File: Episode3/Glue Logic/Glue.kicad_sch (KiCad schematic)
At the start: 17 parts, among them U10 ATF750C, U11 ATF22V10, U7 ATF22V10C, U8 ATF22V10, U9 ATF750C, X1 16MHz

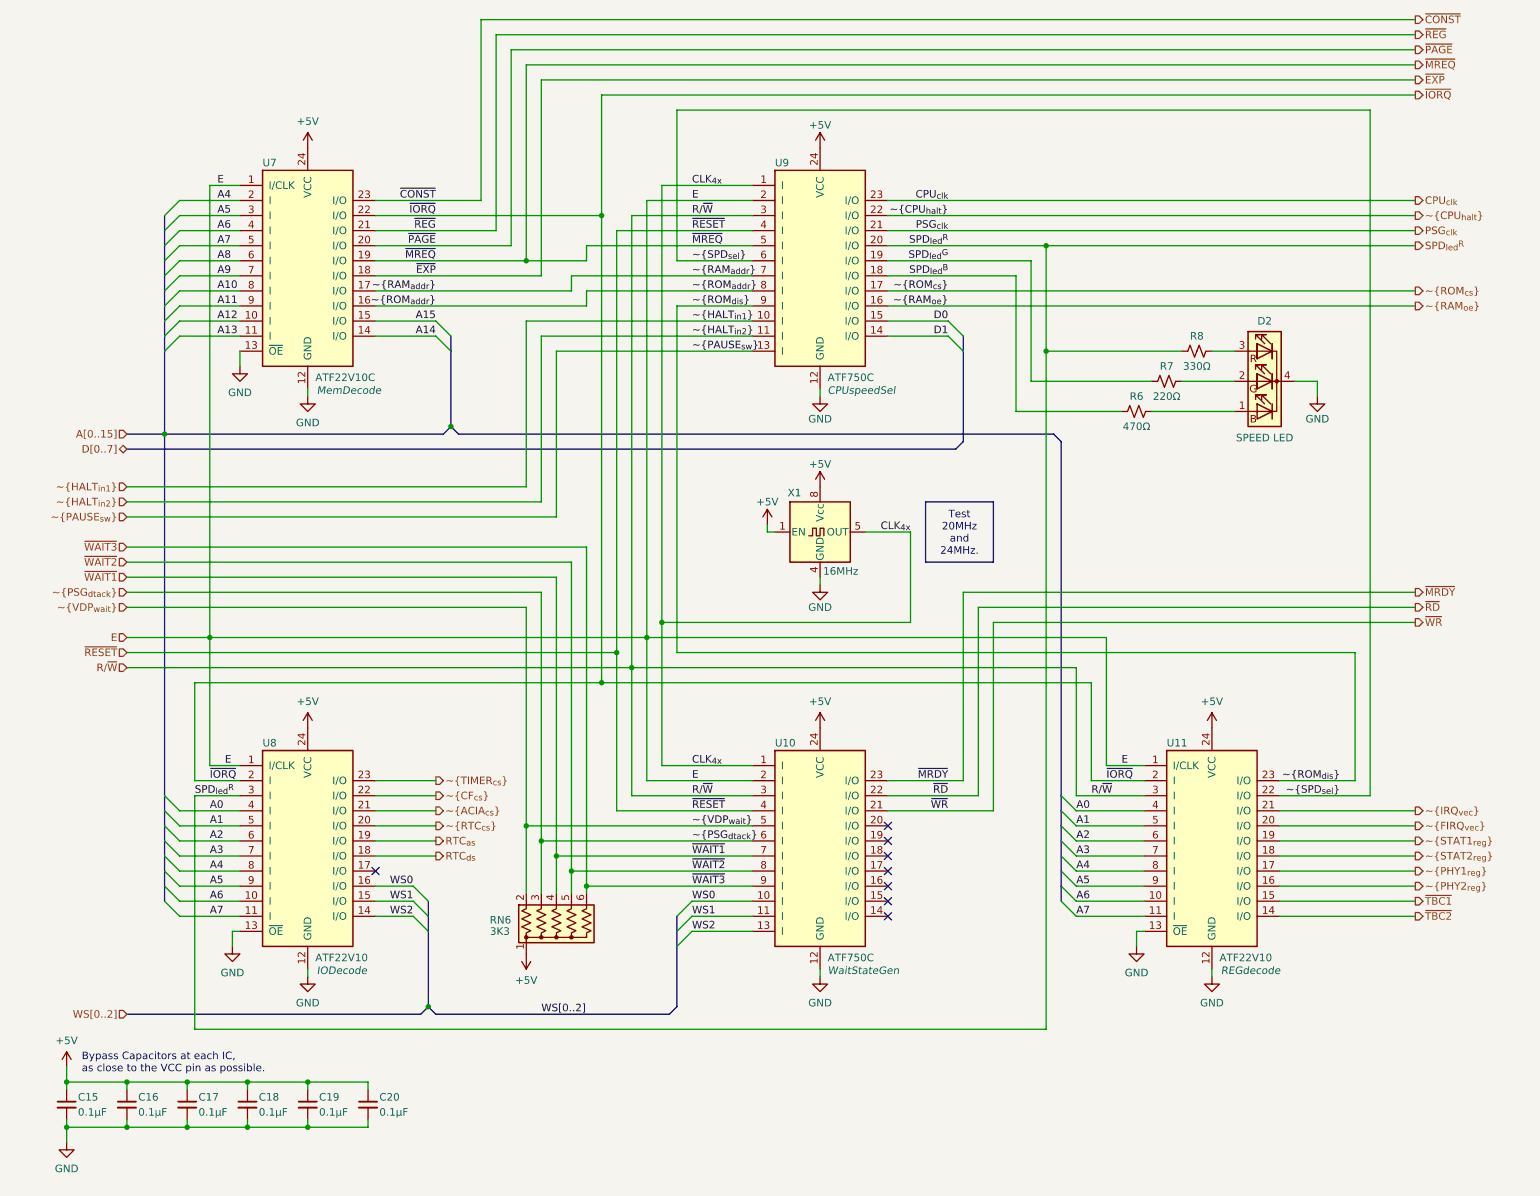
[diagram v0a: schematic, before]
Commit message: Major updates to PLDs
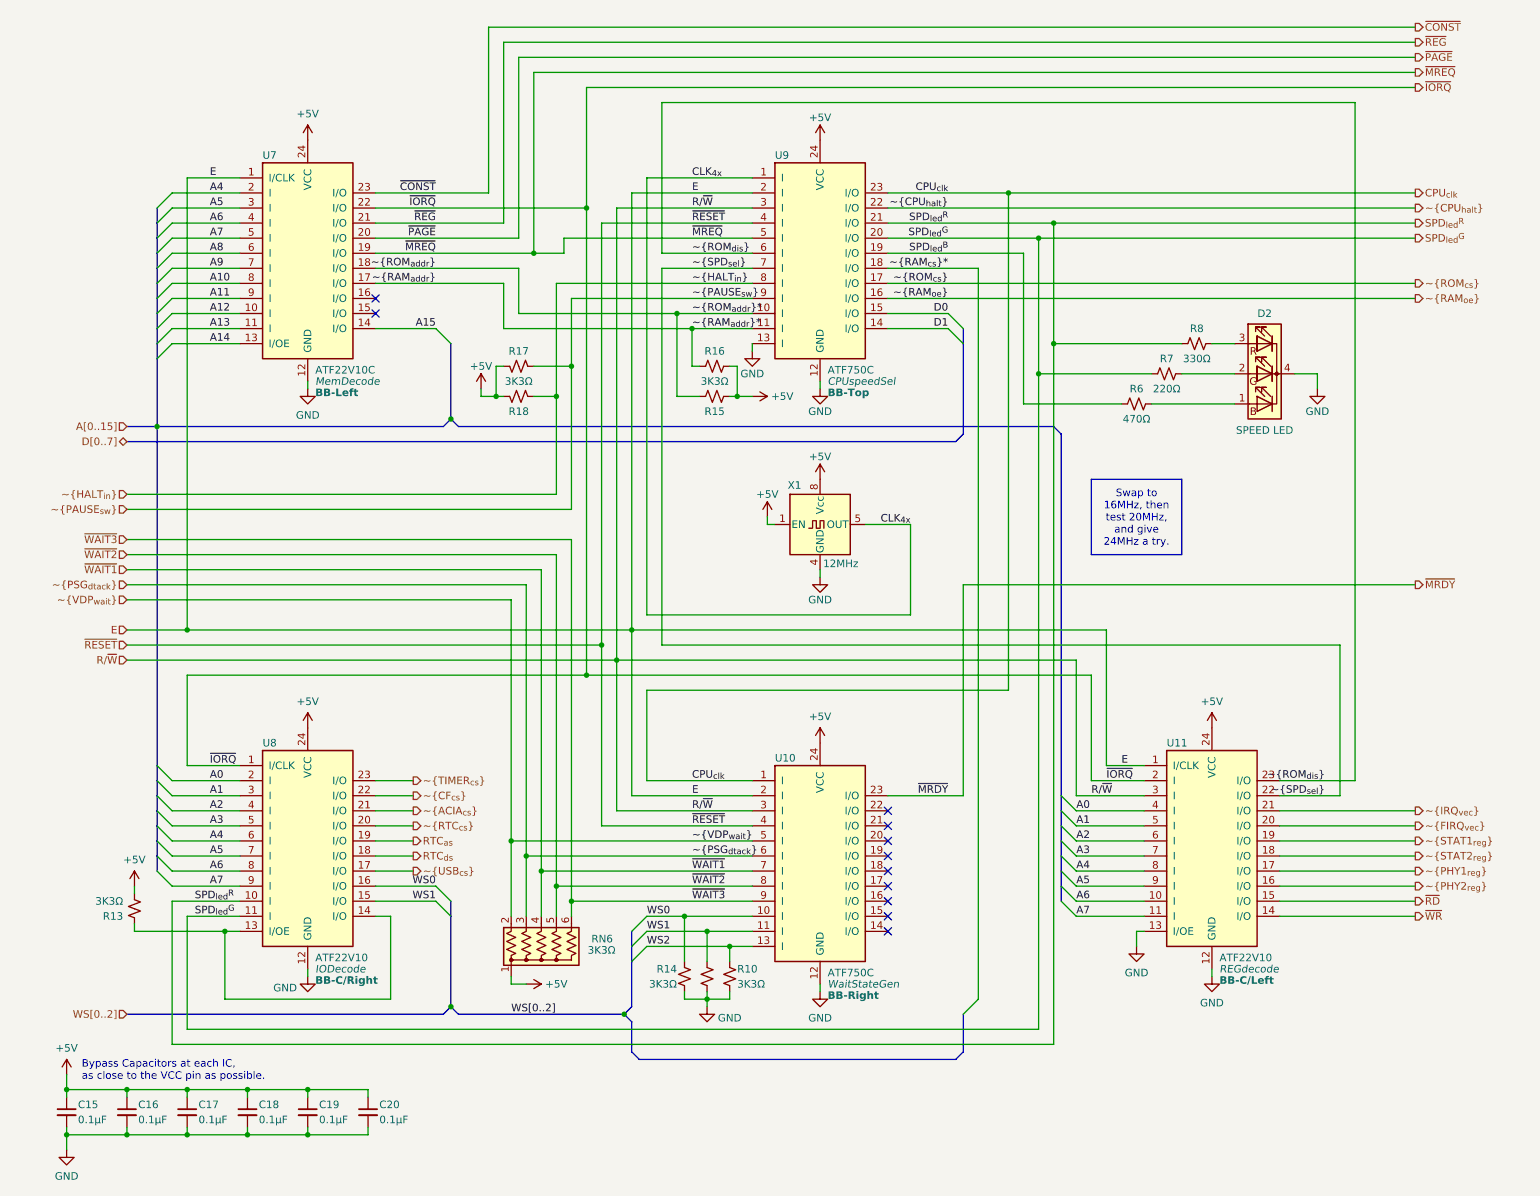
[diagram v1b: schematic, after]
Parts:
- added R10, R13, R14, R15, R16, R17, R18, R9: 3K3Ω, symbol Device:R_Small_US
- RN6: value 3K3 -> 3K3Ω
- U10: Position (none) -> BB-Right
- U11: footprint Package_DIP:DIP-24_W7.62mm_Socket -> Package_DIP:DIP-24_W7.62mm_Socket_LongPads; Position (none) -> BB-C/Left
- U7: Position (none) -> BB-Left
- U8: footprint Package_DIP:DIP-24_W7.62mm_Socket -> Package_DIP:DIP-24_W7.62mm_Socket_LongPads; Position (none) -> BB-C/Right
- U9: Position (none) -> BB-Top
- X1: value 16MHz -> 12MHz
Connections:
- net PSG_{clk} is gone; now on net SPD_{led}^{R}: U9.21 (I/O)
- net ~{EXP} is gone; now on net ~{ROM_{addr}}: U7.18 (I/O)
- net ~{HALT_{in1}} is gone; now on net ~{ROM_{addr}}: U9.10 (I)
- net ~{HALT_{in2}} is gone; now on net ~{RAM_{addr}}: U9.11 (I)
- net ~{TBC1} is gone; now on net ~{RD}: U11.15 (I/O)
- net ~{TBC2} is gone; now on net ~{WR}: U11.14 (I/O)
- net +5V: now also R13.1, R15.1, R16.1, R17.1, R18.1
- net A0: now also U8.2 (I); no longer U8.4 (I)
- net A1: now also U8.3 (I); no longer U8.5 (I)
- net A14: now also U7.13 (I/OE); no longer U7.14 (I/O)
- net A15: now also U7.14 (I/O); no longer U7.15 (I/O)
- net A2: now also U8.4 (I); no longer U8.6 (I)
- net A3: now also U8.5 (I); no longer U8.7 (I)
- net A4: now also U8.6 (I); no longer U8.8 (I)
- net A5: now also U8.7 (I); no longer U8.9 (I)
- net A6: now also U8.8 (I); no longer U8.10 (I)
- net A7: now also U8.9 (I); no longer U8.11 (I)
- net CLK_{4x}: no longer U10.1 (I)
- net CPU_{clk}: now also U10.1 (I)
- net E: no longer U8.1 (I/CLK)
- net GND: now also U9.13 (I), R10.1, R14.1, R9.1; no longer U7.13 (~{OE}), U8.13 (~{OE})
- net SPD_{led}^{B}: now also U9.19 (I/O); no longer U9.18 (I/O)
- net SPD_{led}^{G}: now also U8.11 (I), U9.20 (I/O); no longer U9.19 (I/O)
- net SPD_{led}^{R}: now also U8.10 (I); no longer U8.3 (I), U9.20 (I/O)
- net WS0: now also R14.2
- net WS1: now also R9.2
- net WS2: now also R10.2; no longer U8.14 (I/O)
- net ~{IORQ}: now also U8.1 (I/CLK); no longer U8.2 (I)
- net ~{PAUSE_{sw}}: now also U9.9 (I), R17.2; no longer U9.13 (I)
- net ~{RAM_{addr}}: now also R16.2; no longer U9.7 (I)
- net ~{RD}: no longer U10.22 (I/O)
- net ~{ROM_{addr}}: now also R15.2; no longer U7.16 (I/O), U9.8 (I)
- net ~{ROM_{dis}}: now also U9.6 (I); no longer U9.9 (I)
- net ~{SPD_{sel}}: now also U9.7 (I); no longer U9.6 (I)
- net ~{WR}: no longer U10.21 (I/O)
- net ~{USB_{cs}}: now reaches U8.17 (I/O)
- new net: R13.2, U8.13 (I/OE), U8.14 (I/O)
- new net ~{HALT_{in}}: R18.2, U9.8 (I)
- new net ~{RAM_{cs}}*: U9.18 (I/O)
- no-connect marks 8 -> 11
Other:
- moved on the sheet: C15, C16, C17, C18, C19, C20, D2, R6, R7, R8, RN6, U10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
